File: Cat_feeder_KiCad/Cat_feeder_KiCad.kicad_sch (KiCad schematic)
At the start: 12 parts, among them J1 Conn_01x03_Pin, J2 Conn_01x04_Pin, SW1 SW_Push, SW2 Reset button, U1 ESP32-S3-WROOM-1, U3 ER_OLEDM0.91_1x-I2C, U4 LD1117V33

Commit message: changing schematic bc I was dumb yesterday
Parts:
- removed U3: ER_OLEDM0.91_1x-I2C, Display:ER_OLEDM0.91_1x-I2C, symbol Display_Graphic:ER_OLEDM0.91_1x-I2C
- added BT1: Battery_Cell, symbol Device:Battery_Cell
- added C5: 100nF, Capacitor_SMD:C_0805_2012Metric, symbol Device:C
- added D1: 1N4148, Diode_THT:D_DO-35_SOD27_P7.62mm_Horizontal, symbol Diode:1N4148
- added R1: 100Ω, Resistor_SMD:R_0805_2012Metric, symbol Device:R
- added U5: DS3231M, Package_SO:SOIC-16W_7.5x10.3mm_P1.27mm, symbol Timer_RTC:DS3231M
- J2: footprint (none) -> Connector_PinHeader_2.54mm:PinHeader_1x04_P2.54mm_Vertical
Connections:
- net SCL_IO18 is gone; now on net SDA: U1.11 (IO18)
- net SDA_IO21 is gone; now on net SCL: U1.23 (IO21)
- net +3.3V: now also U5.2 (VCC)
- net GND: now also BT1.2 (-), C5.2, U5.10 (GND), U5.11 (GND), U5.12 (GND), U5.13 (GND), U5.5 (GND), U5.6 (GND), U5.7 (GND), U5.8 (GND), U5.9 (GND)
- net SCL: now also J2.3 (Pin_3); no longer J2.4 (Pin_4)
- net SDA: now also J2.4 (Pin_4); no longer J2.3 (Pin_3)
- net SDA_IO: now reaches U1.27 (IO0)
- net SDA_IO: now also U5.15 (SDA)
- net SCL_I0: now reaches U1.39 (IO1)
- net SCL_I0: now also U5.16 (SCL)
- net RTC_board/SCL: no longer names the net of U1.18 (IO10)
- net RTC_board/SDA: no longer names the net of U1.19 (IO11)
- new net: C5.1, D1.1 (K), U5.14 (VBAT)
- new net: D1.2 (A), R1.1
- new net: BT1.1 (+), R1.2
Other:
- removed sheet RTC_board
- moved on the sheet: J2

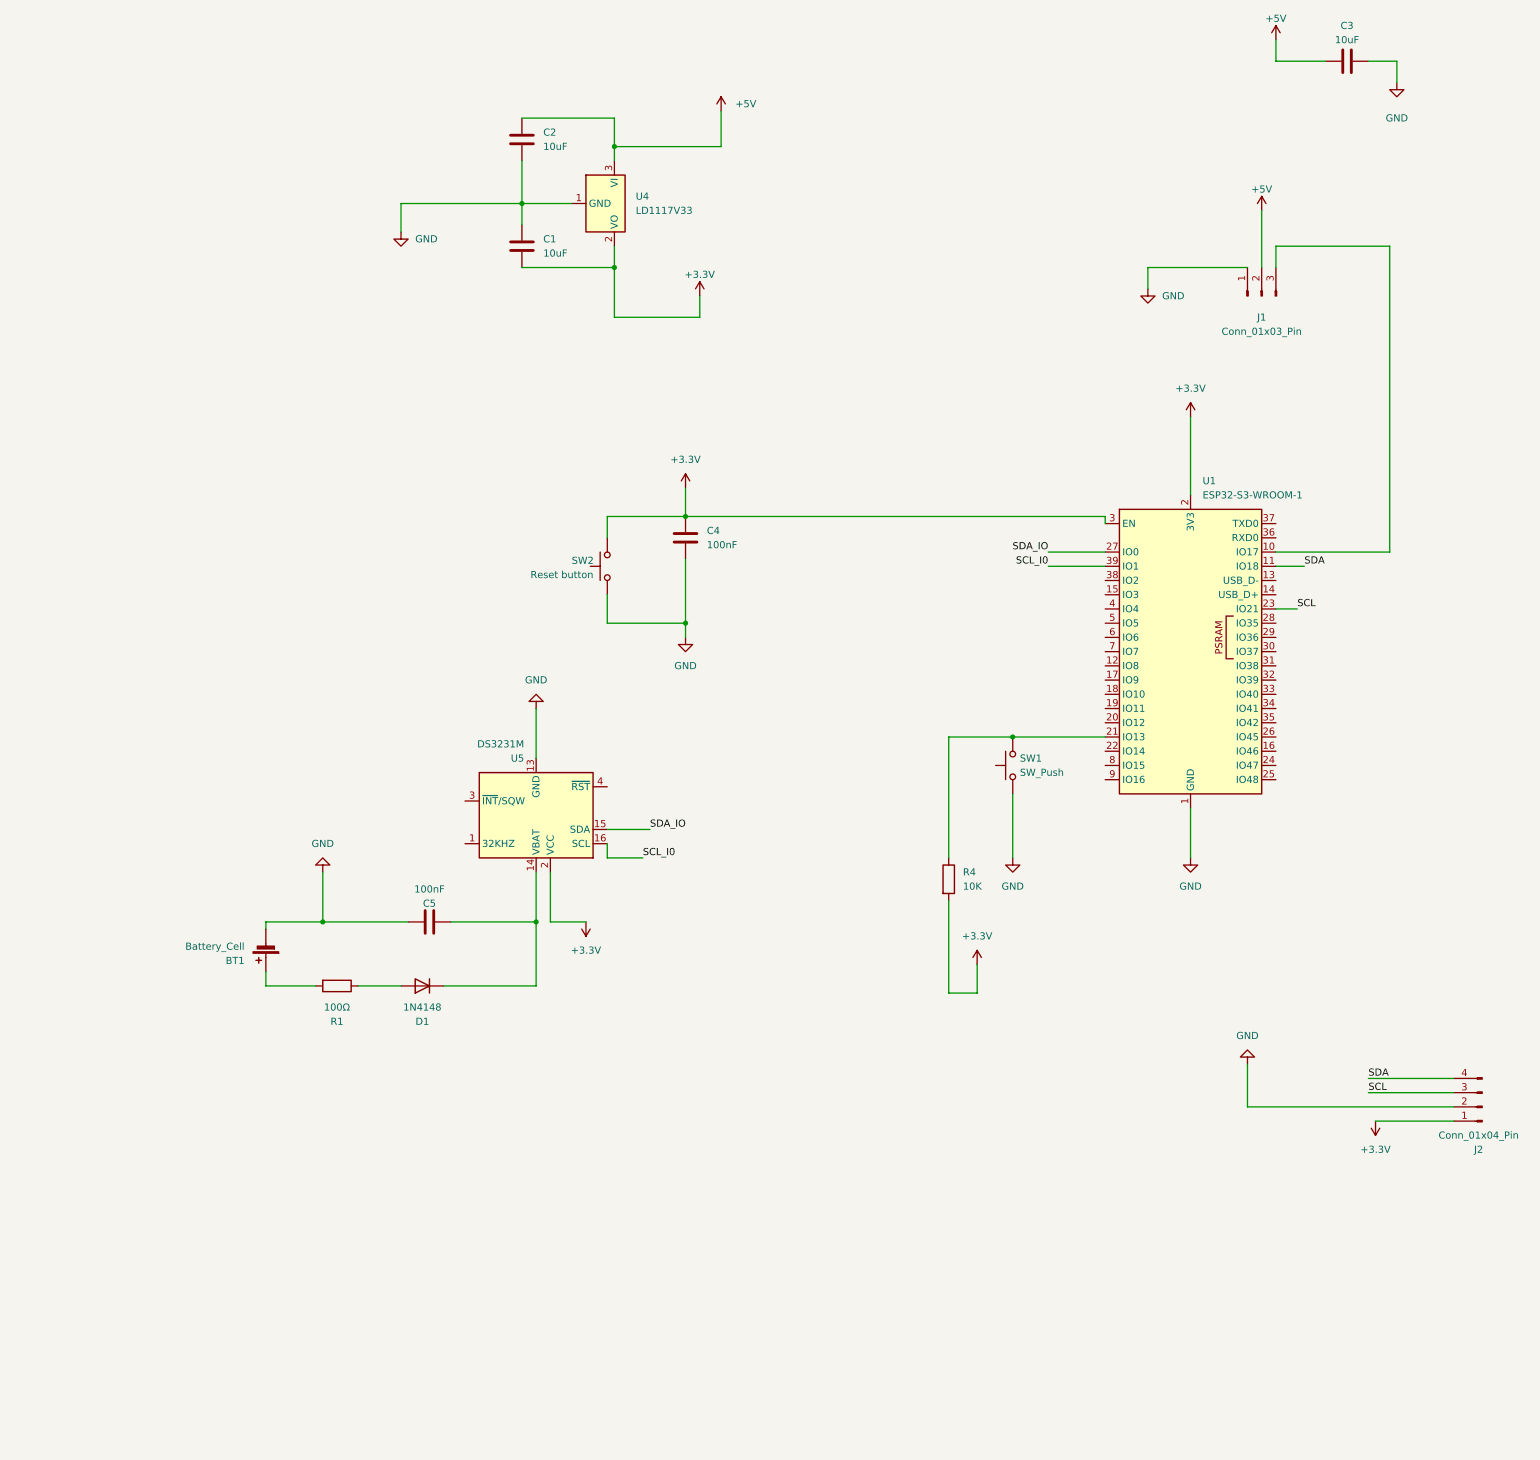
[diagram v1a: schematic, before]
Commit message: doing schematic
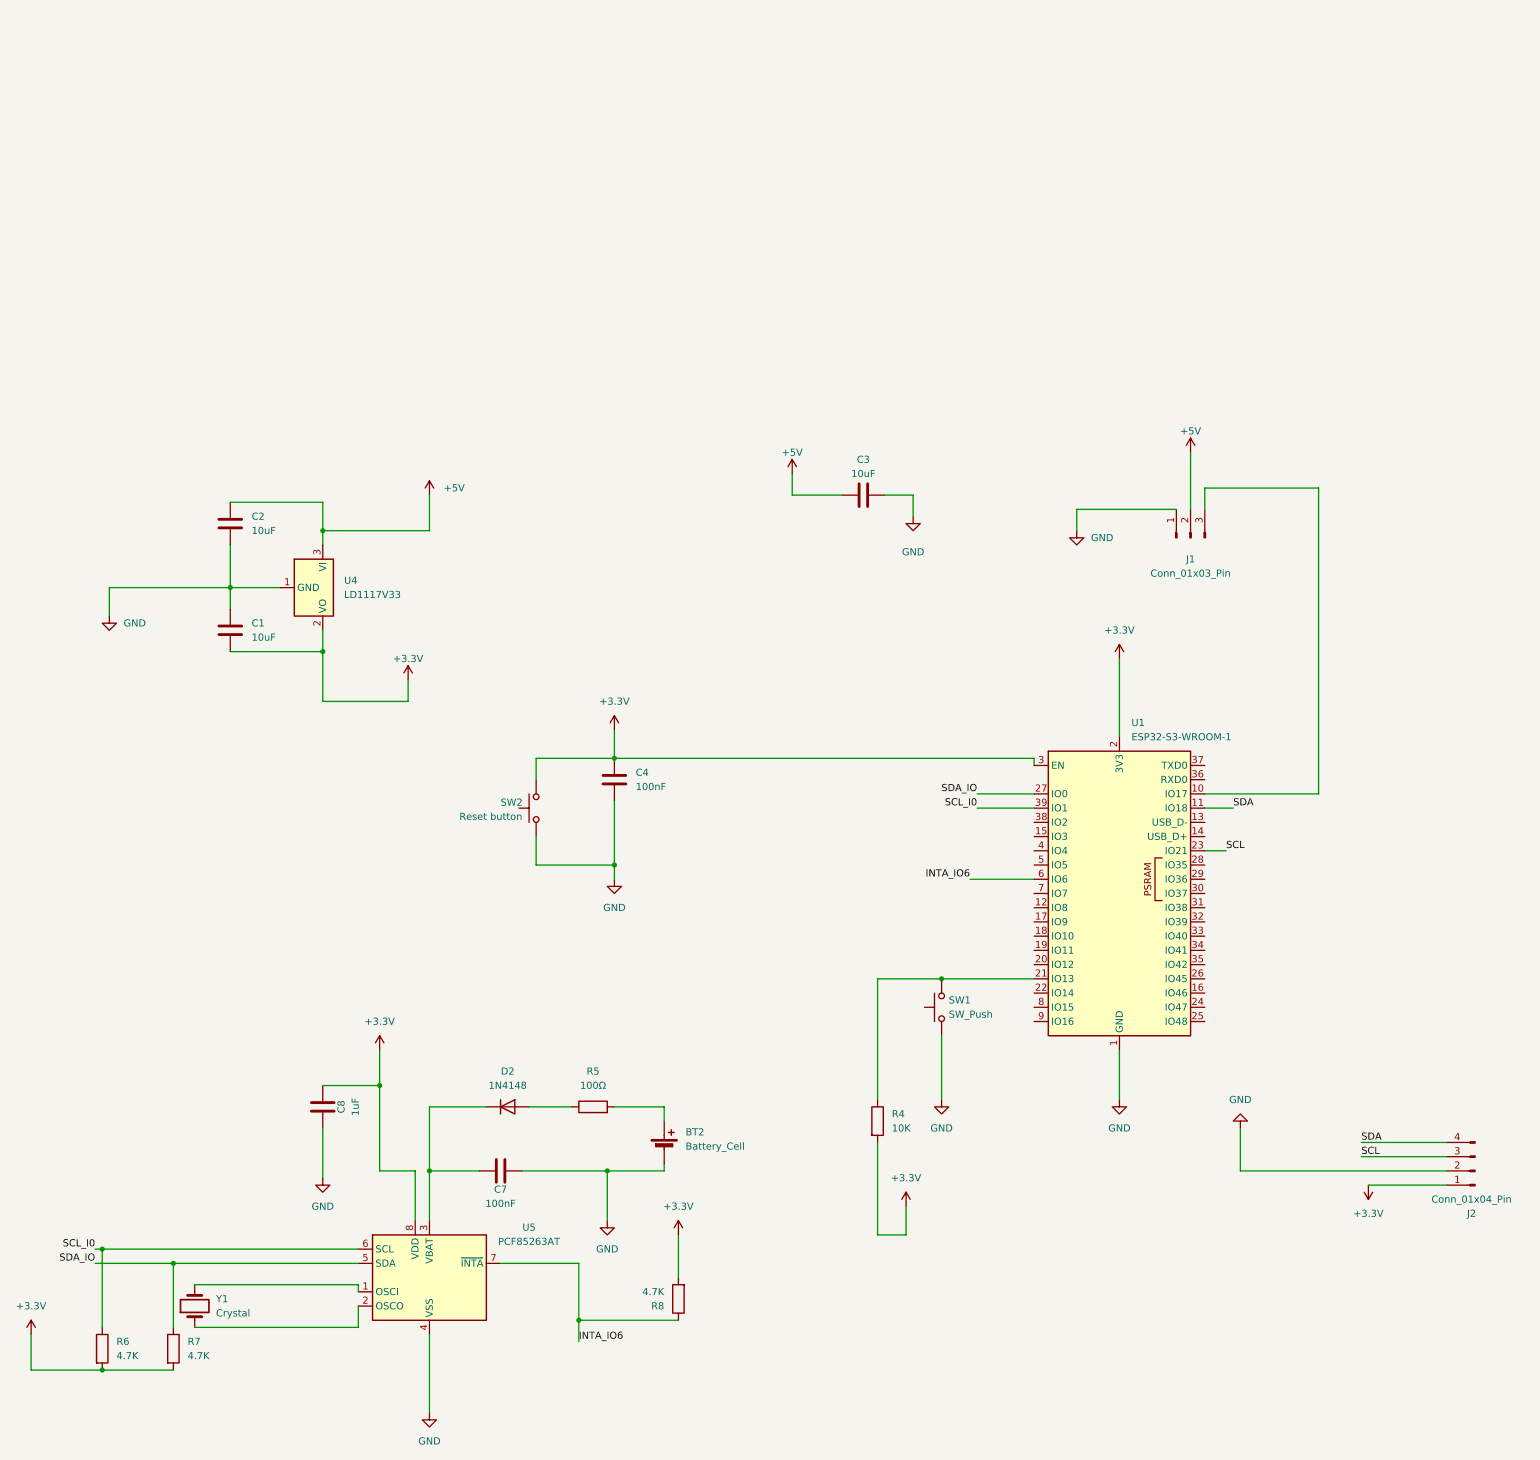
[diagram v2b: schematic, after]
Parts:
- removed BT1: Battery_Cell, symbol Device:Battery_Cell
- removed C5: 100nF, Capacitor_SMD:C_0805_2012Metric, symbol Device:C
- removed D1: 1N4148, Diode_THT:D_DO-35_SOD27_P7.62mm_Horizontal, symbol Diode:1N4148
- removed R1: 100Ω, Resistor_SMD:R_0805_2012Metric, symbol Device:R
- removed U5: DS3231M, Package_SO:SOIC-16W_7.5x10.3mm_P1.27mm, symbol Timer_RTC:DS3231M
- added BT2: Battery_Cell, symbol Device:Battery_Cell
- added C7: 100nF, Capacitor_SMD:C_0805_2012Metric, symbol Device:C
- added C8: 1uF, Capacitor_SMD:C_0805_2012Metric, symbol Device:C
- added D2: 1N4148, Diode_THT:D_DO-35_SOD27_P7.62mm_Horizontal, symbol Diode:1N4148
- added R5: 100Ω, Resistor_SMD:R_0805_2012Metric, symbol Device:R
- added R6, R7, R8: 4.7K, symbol Device:R
- added U5: PCF85263AT, Package_SO:SOIC-8_3.9x4.9mm_P1.27mm, symbol Timer_RTC:PCF85263AT
- added Y1: Crystal, symbol Device:Crystal
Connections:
- net +3.3V: now also C8.2, R6.2, R7.2, R8.2, U5.8 (VDD)
- net GND: now also BT2.2 (-), C7.2, C8.1, U5.4 (VSS)
- net SCL_I0: now also R6.1, U5.6 (SCL)
- net SDA_IO: now also R7.1, U5.5 (SDA)
- net INTA_IO6: now reaches U1.6 (IO6)
- net INTA_IO6: now also R8.1, U5.7 (~{INTA})
- new net: C7.1, D2.1 (K), U5.3 (VBAT)
- new net: D2.2 (A), R5.1
- new net: U5.2 (OSCO), Y1.1
- new net: U5.1 (OSCI), Y1.2
- new net: BT2.1 (+), R5.2
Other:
- moved on the sheet: C1, C2, C3, C4, J1, J2, R4, SW1, SW2, U1, U4

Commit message: adding footprints
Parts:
- BT2: footprint (none) -> Battery:BatteryHolder_Keystone_3034_1x20mm
- R6, R7, R8: footprint (none) -> Resistor_SMD:R_0805_2012Metric
- Y1: footprint (none) -> Crystal:Crystal_SMD_3225-4Pin_3.2x2.5mm
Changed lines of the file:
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@@
 			)
 		)
-		(property "Footprint" ""
+		(property "Footprint" "Resistor_SMD:R_0805_2012Metric"
 			(at 26.162 180.34 90)
 			(hide yes)
@@
 			)
 		)
-		(property "Footprint" ""
+		(property "Footprint" "Crystal:Crystal_SMD_3225-4Pin_3.2x2.5mm"
 			(at 44.45 172.72 0)
 			(hide yes)
@@
 			)
 		)
-		(property "Footprint" ""
+		(property "Footprint" "Resistor_SMD:R_0805_2012Metric"
 			(at 132.588 171.45 90)
 			(hide yes)
@@
 			)
 		)
-		(property "Footprint" ""
+		(property "Footprint" "Battery:BatteryHolder_Keystone_3034_1x20mm"
 			(at 128.27 143.256 90)
 			(hide yes)
@@
 			)
 		)
-		(property "Footprint" ""
+		(property "Footprint" "Resistor_SMD:R_0805_2012Metric"
 			(at 38.862 180.34 90)
 			(hide yes)

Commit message: some schematic work + kicad crashed
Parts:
- Y1: footprint Crystal:Crystal_SMD_3225-4Pin_3.2x2.5mm -> Crystal:Crystal_SMD_0603-2Pin_6.0x3.5mm
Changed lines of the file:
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@@
 			)
 		)
-		(property "Footprint" "Crystal:Crystal_SMD_3225-4Pin_3.2x2.5mm"
+		(property "Footprint" "Crystal:Crystal_SMD_0603-2Pin_6.0x3.5mm"
 			(at 44.45 172.72 0)
 			(hide yes)
